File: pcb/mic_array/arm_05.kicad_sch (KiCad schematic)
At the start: 16 parts, among them U41 IM72D128V01XTMA1, U42 IM72D128V01XTMA1, U43 IM72D128V01XTMA1, U44 IM72D128V01XTMA1, U45 IM72D128V01XTMA1, U46 IM72D128V01XTMA1, U47 IM72D128V01XTMA1, U48 IM72D128V01XTMA1

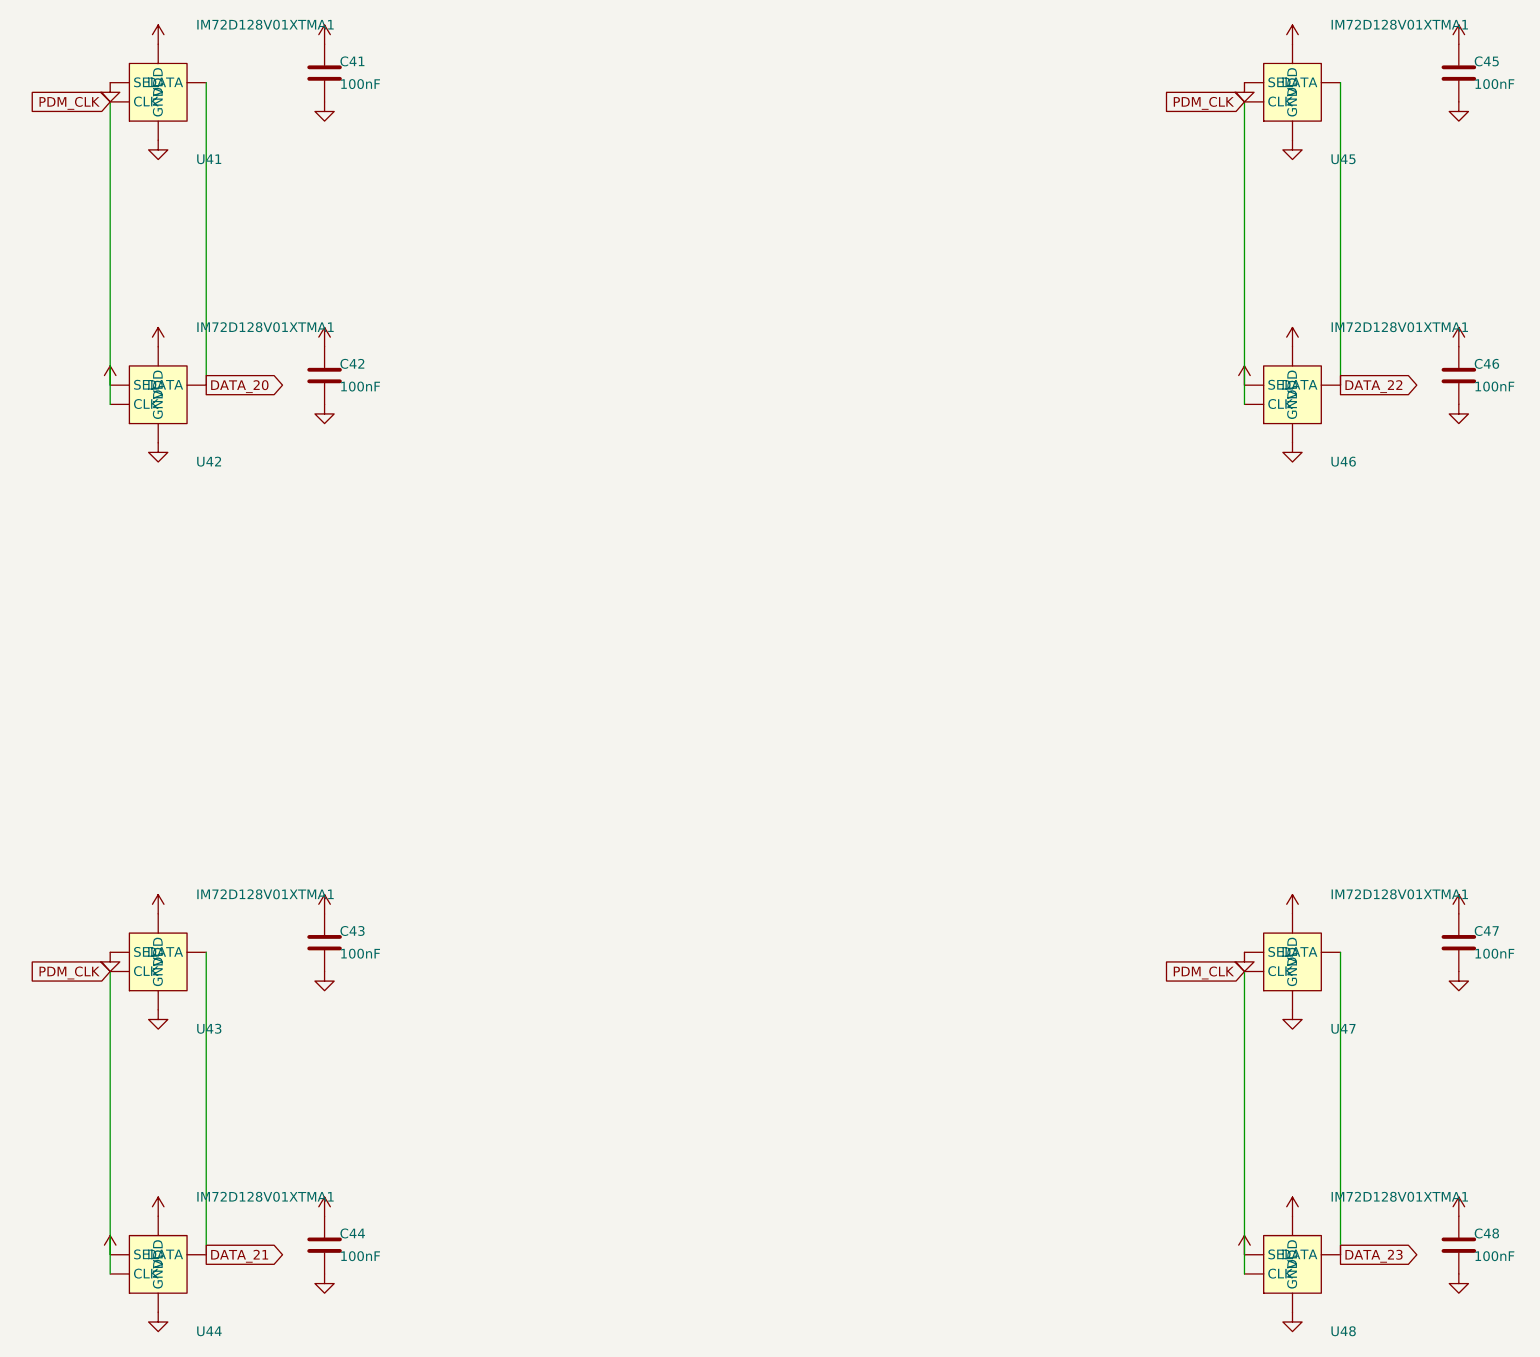
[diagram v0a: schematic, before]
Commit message: Updated.
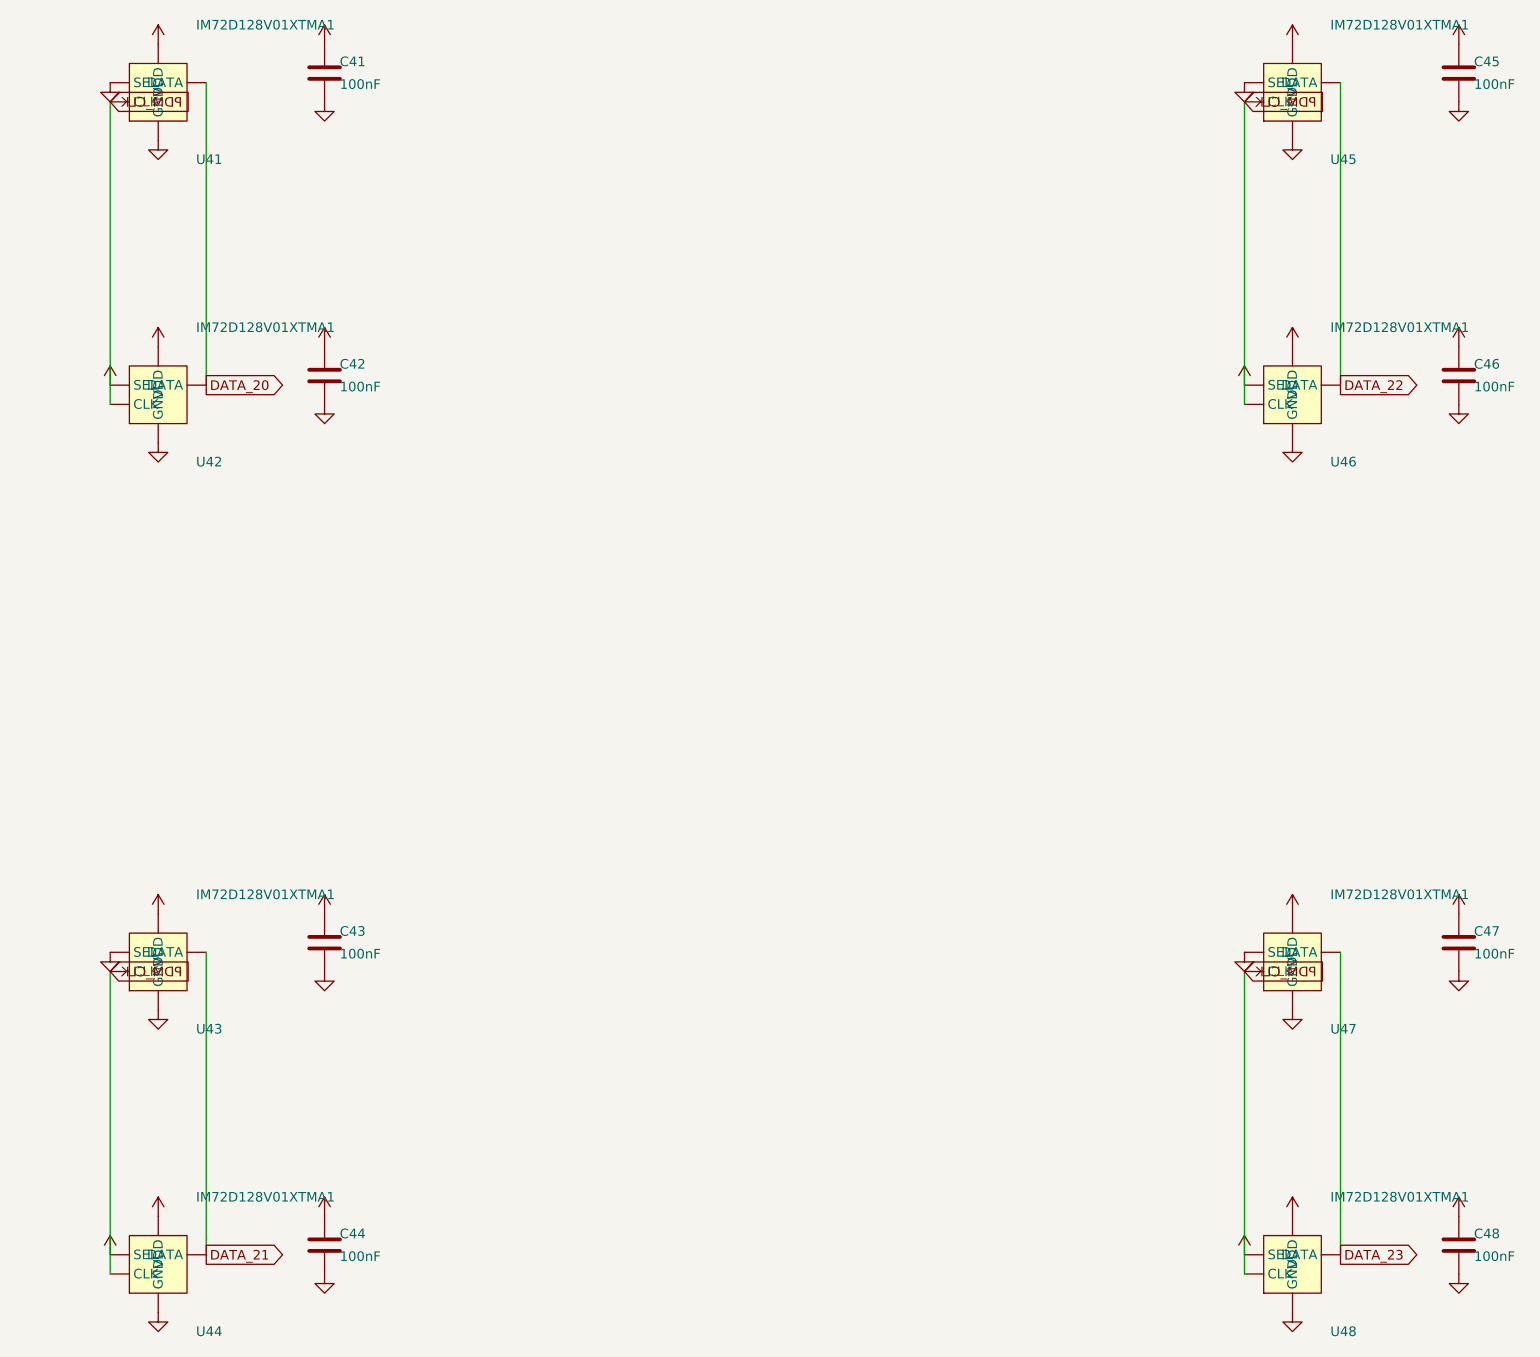
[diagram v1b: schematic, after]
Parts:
- C41, C42, C43, C44, C45, C46, C47, C48: footprint Capacitor_SMD:C_0402_1005Metric -> (none)
- U41, U42, U43, U44, U45, U46, U47, U48: footprint Sensor_Audio:Infineon_PG-LLGA-5-2 -> (none)
